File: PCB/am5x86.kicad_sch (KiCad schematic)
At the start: 45 parts

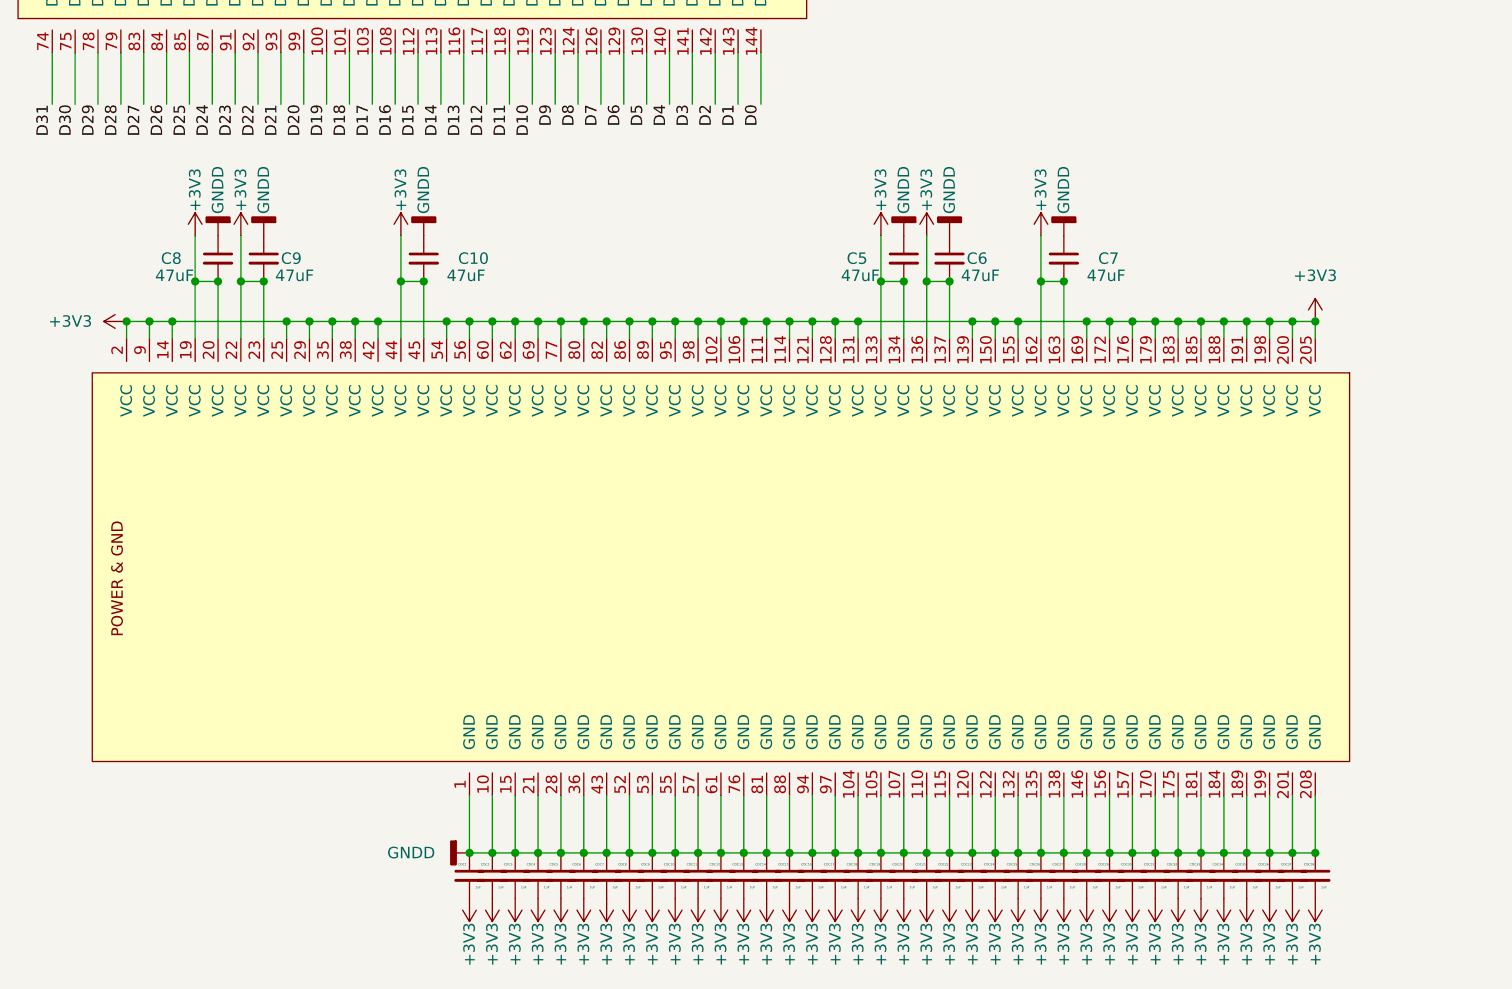
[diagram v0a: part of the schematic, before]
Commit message: progress
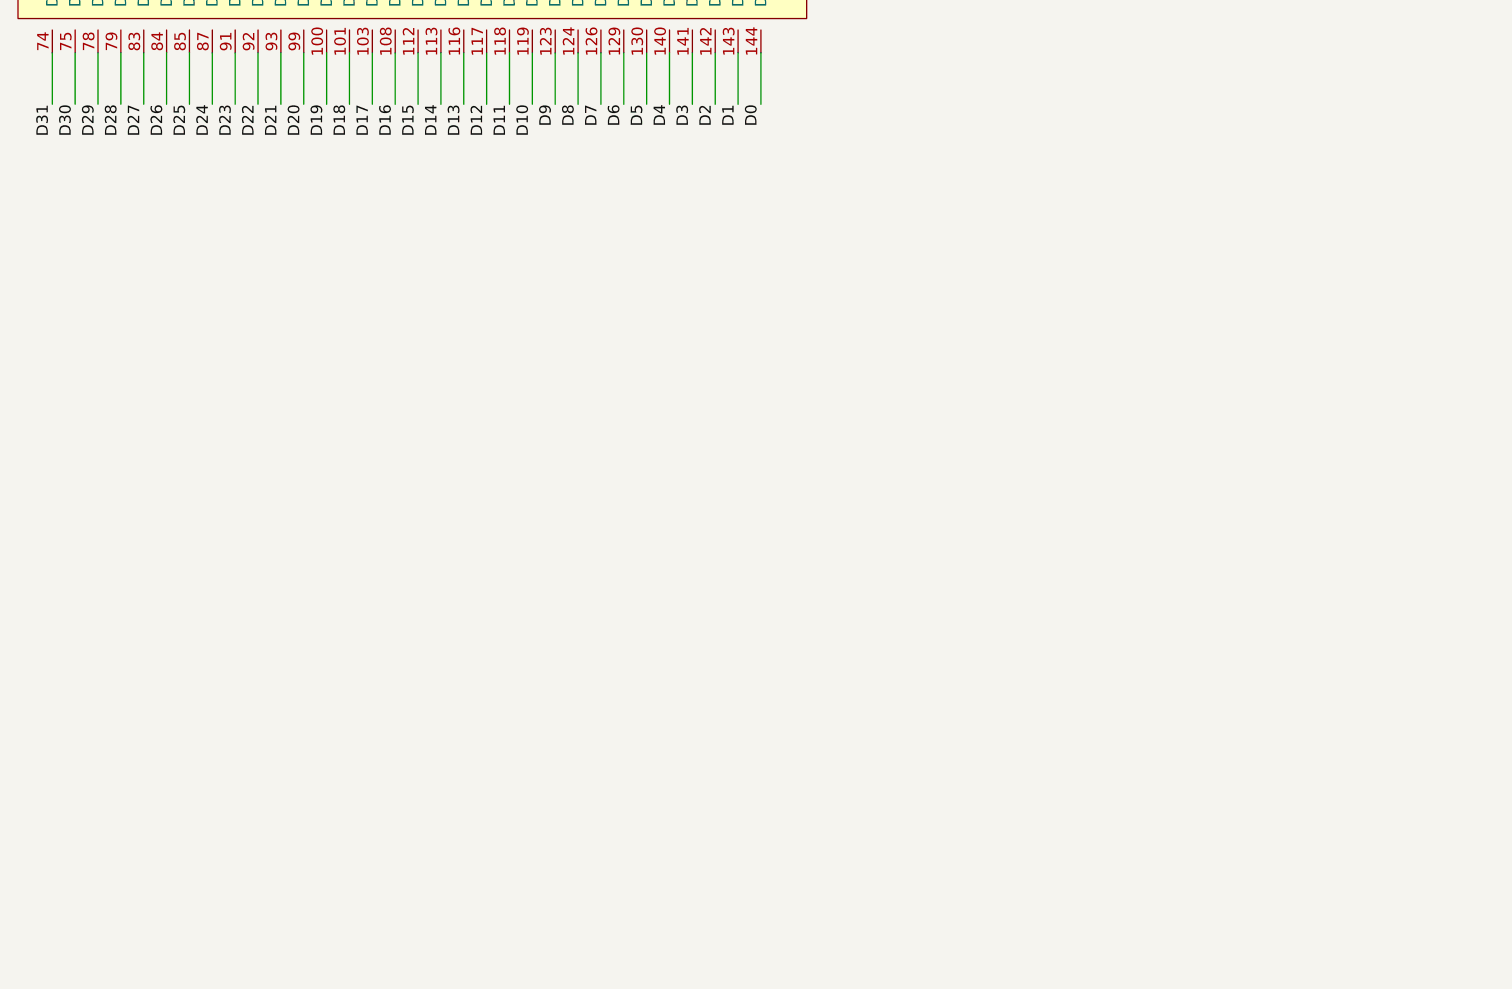
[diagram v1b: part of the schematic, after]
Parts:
- removed C10, C5, C6, C7, C8, C9: 47uF, Capacitor_SMD:C_0603_1608Metric, symbol Device:C_Small
- removed CDC1, CDC10, CDC11, CDC12, CDC13, CDC14, CDC15, CDC16, CDC17, CDC18, CDC19, CDC2, CDC20, CDC21, CDC22, CDC23, CDC24, CDC25, CDC26, CDC27, CDC28, CDC29, CDC3, CDC30, CDC31, CDC32, CDC33, CDC34, CDC35, CDC36, CDC37, CDC38, CDC4, CDC5, CDC6, CDC7, CDC8, CDC9: 1uF, Capacitor_SMD:C_0402_1005Metric, symbol Device:C_Small
- removed unit 1 of U3
- U3: value (none) -> AM5x86 PQFP208

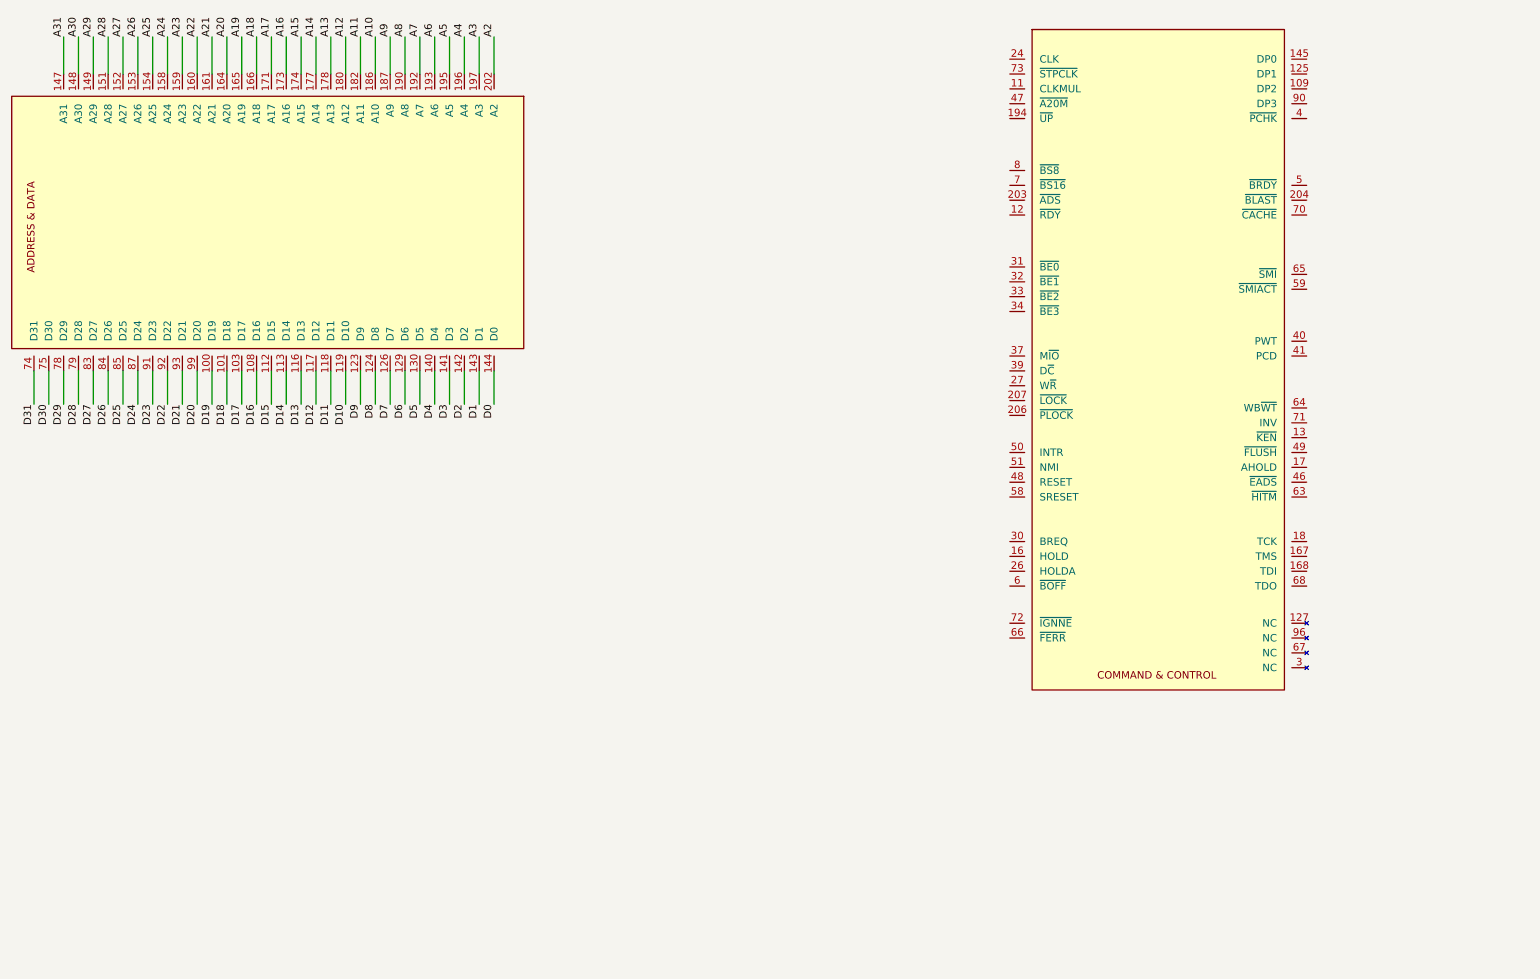
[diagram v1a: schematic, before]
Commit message: more progress
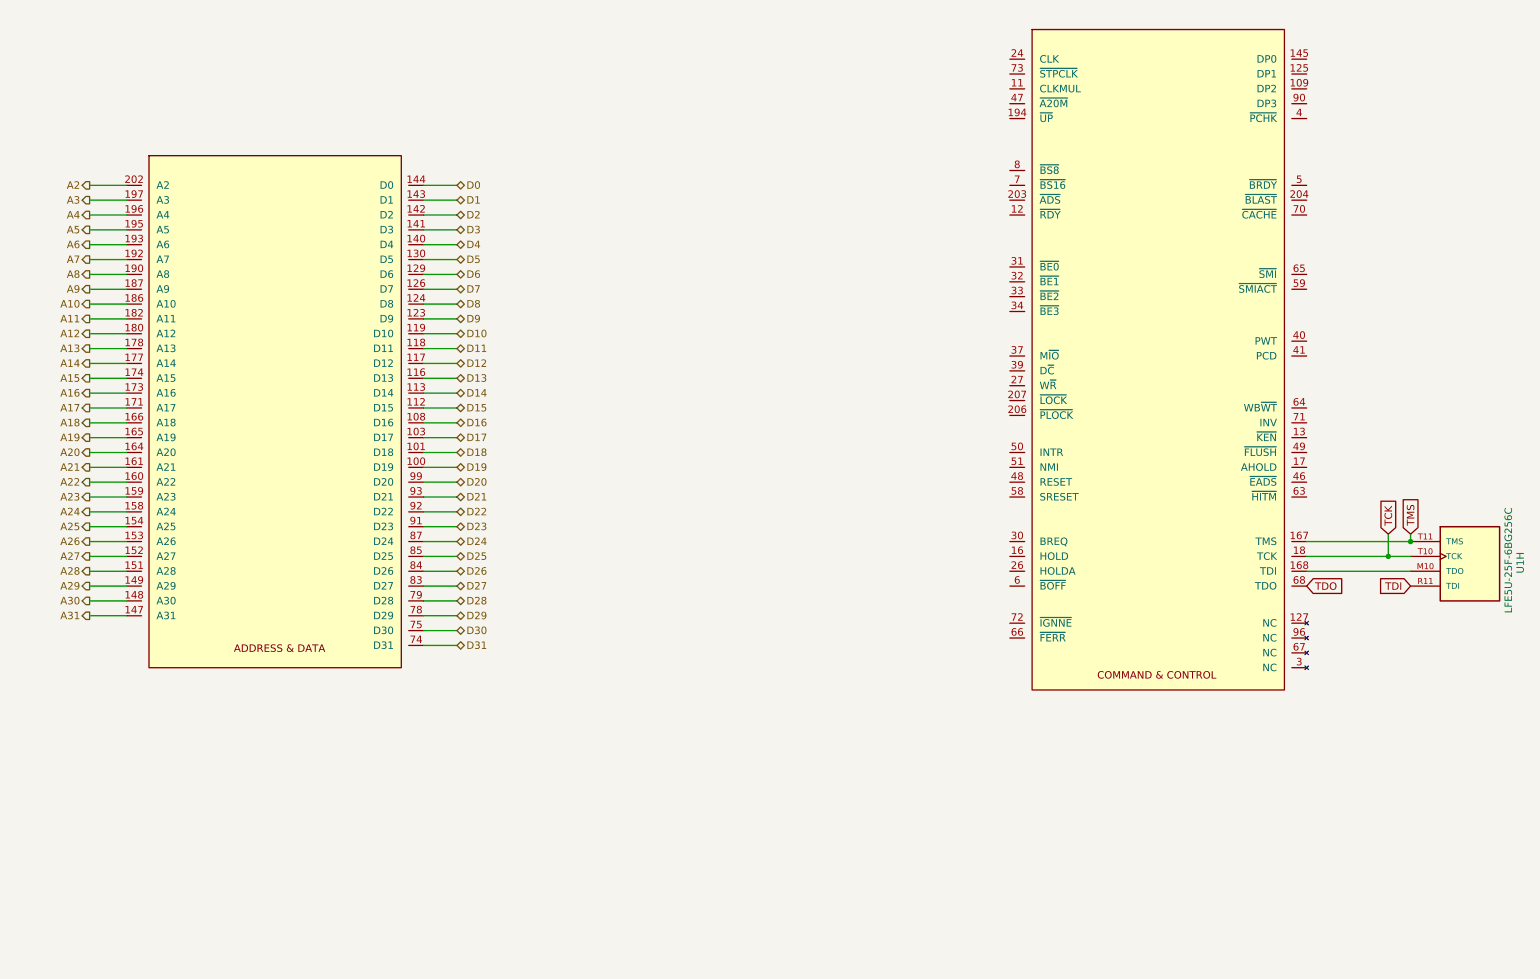
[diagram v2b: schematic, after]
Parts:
- added U1: LFE5U-25F-6BG256C, ECP5:BGA256C80P16X16_1400X1400X170, symbol Lattice:LFE5U-25F-6BG256C
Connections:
- net TMS: now reaches U3.167 (TMS)
- net TMS: now also U1.T11 (TMS)
- net at U3.168 (TDI): now also U1.M10 (TDO)
- net TCK: now reaches U3.18 (TCK)
- net TCK: now also U1.T10 (TCK)
- net TDO: now reaches U3.68 (TDO)
- new net TDI: U1.R11 (TDI)
